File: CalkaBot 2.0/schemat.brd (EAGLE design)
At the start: 94.4 x 101.8 mm, 55 parts, among them IC1 TB6612FNG, IC2 LM339D, IC3 7806DT, Q1 16MHz, X1 MINI-USB-32005-301

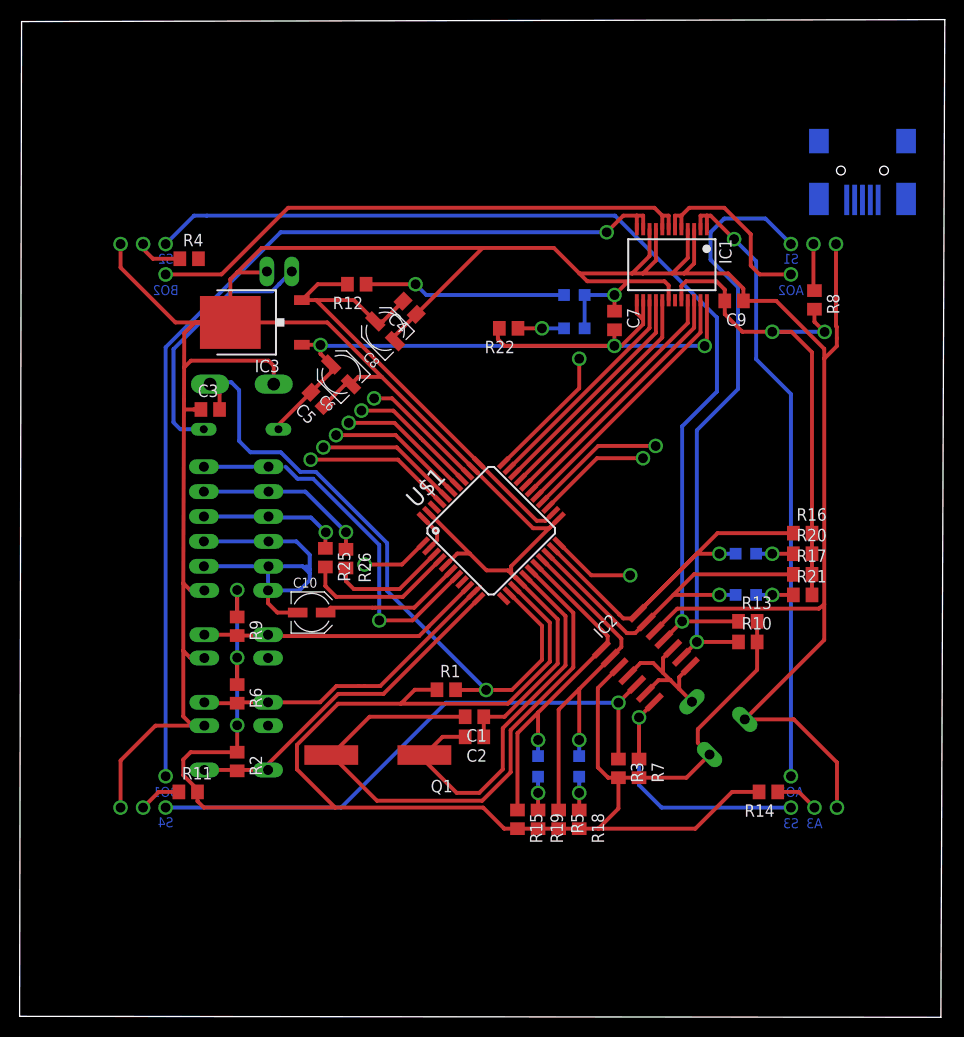
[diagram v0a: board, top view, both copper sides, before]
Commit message: zmiana przycisków
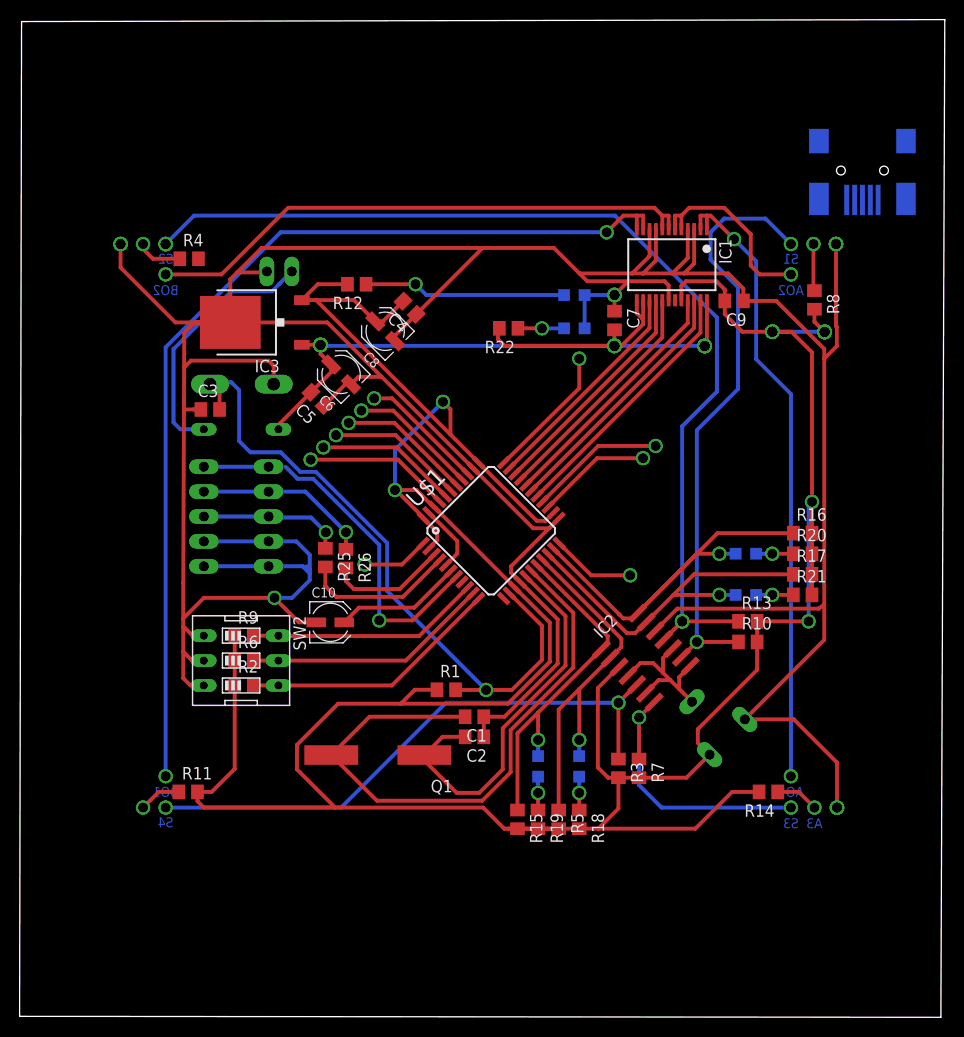
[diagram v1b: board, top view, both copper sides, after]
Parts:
- removed BUT1, BUT2, BUT3: (no value), switch-omron:B3F-10XX
- added SW2: (no value), special:EDG-03
- moved R2 7.83 mm to (25.0, 22.7), turned to 0 degrees
- moved R6 3.47 mm to (25.0, 25.2), turned to 0 degrees
- moved C10 2.15 mm to (33.8, 29.1)
- moved R9 1.22 mm to (25.0, 27.7), turned to 0 degrees
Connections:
- net GND: now also SW2.1, SW2.2, SW2.3; no longer BUT1.1, BUT1.2, BUT2.1, BUT2.2, BUT3.1, BUT3.2
- net MISO: now also SW2.4; no longer BUT1.3, BUT1.4
- net MOSI: now also SW2.5; no longer BUT2.3, BUT2.4
- net SCK: now also SW2.6; no longer BUT3.3, BUT3.4
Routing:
- net VCC: track 297.7 -> 342.4 mm, vias 5 -> 12
- net GND: track 446.3 -> 428.0 mm, vias 5 -> 9
- net MISO: track 35.7 -> 26.7 mm
- net MOSI: track 33.1 -> 25.4 mm
- net SCK: track 29.0 -> 24.0 mm
- net UCAP: track 14.6 -> 13.1 mm
- net VM: vias 3 -> 12
- net S4: vias 2 -> 4
